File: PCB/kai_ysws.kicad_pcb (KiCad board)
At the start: 4 copper layers, 22 x 42 mm, 163 parts, among them J1 Bus_M.2_Socket_M, U1 24C02Cx-x-MNY, U2 AP2112K-3.3, U3 AP2112K-1.8, U4 RP23534A, U5 CH382L, Y1 22.1184MHz, Y2 ABM8-272-T3

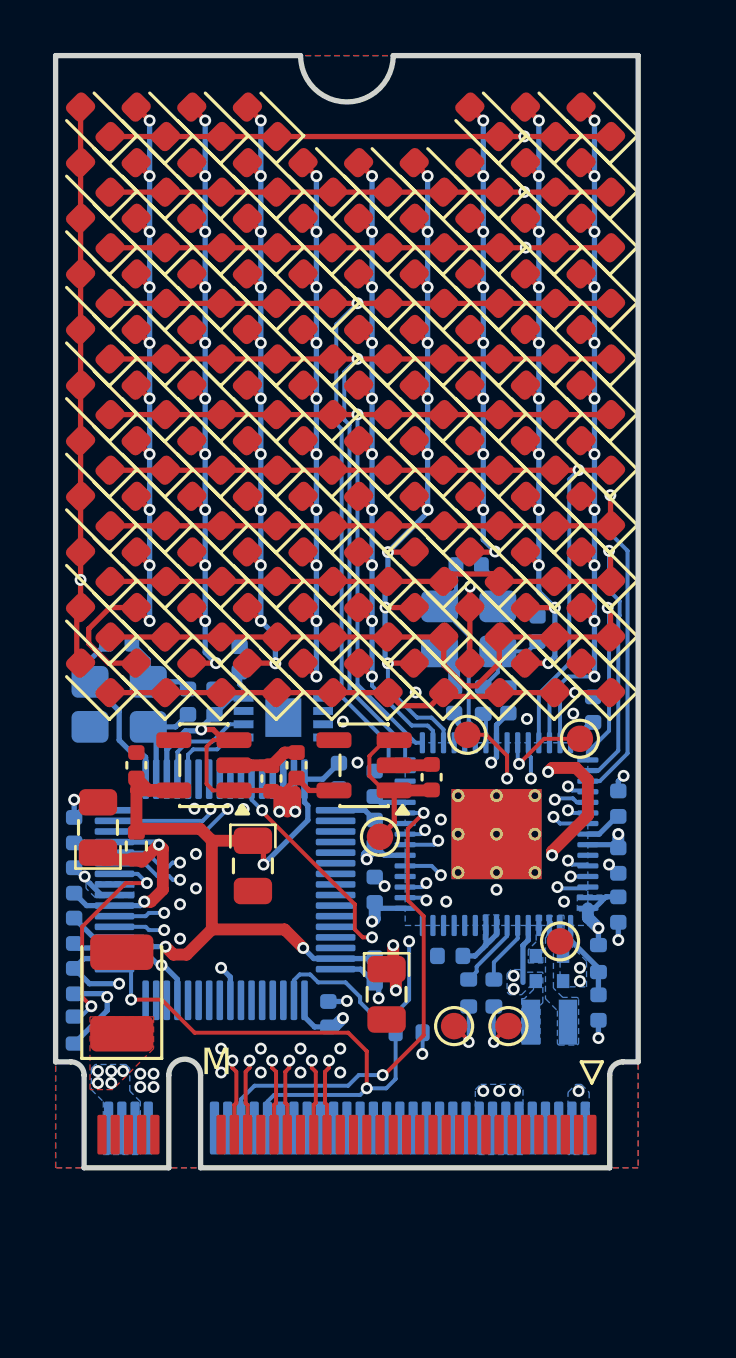
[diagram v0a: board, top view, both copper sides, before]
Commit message: fixed Bom again and small pcb things
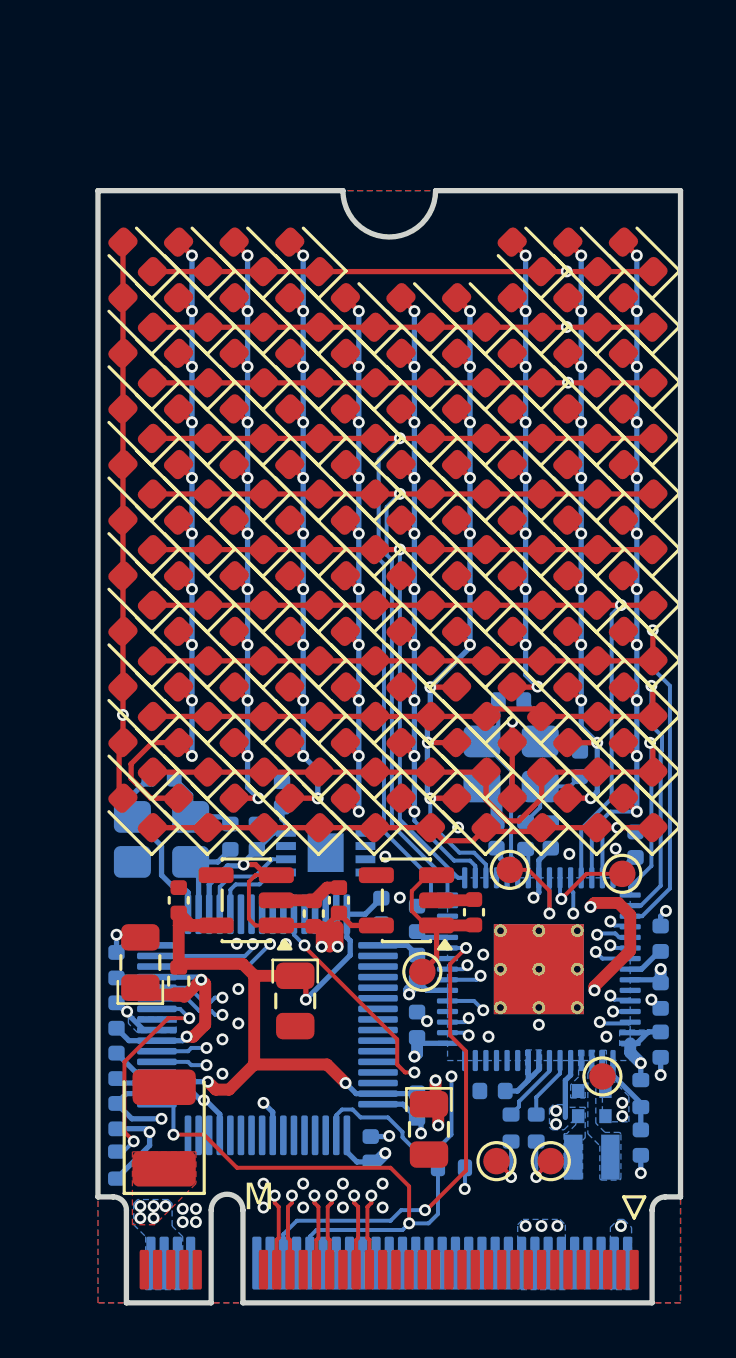
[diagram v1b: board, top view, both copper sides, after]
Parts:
- moved C32 5.35 mm to (135.3, 119.7)
- moved D29 5.35 mm to (133.3, 101.7)
- moved D49 5.35 mm to (133.3, 105.9)
- moved D79 5.35 mm to (133.3, 112.2)
- moved D99 5.35 mm to (133.3, 116.4)
- moved R5 5.35 mm to (131.6, 130.4)
- moved TP2 5.35 mm to (130.1, 131.7)
- moved TP5 5.35 mm to (130.6, 120.7)
- moved C10 5.35 mm to (125.7, 122.2)
- moved C11 5.35 mm to (115.7, 126.2)
- moved C2 5.35 mm to (117.4, 117.2)
- moved C9 5.35 mm to (115.7, 128.1)
- moved D23 5.35 mm to (120.7, 101.7)
- moved D25 5.35 mm to (124.9, 101.7)
- moved D43 5.35 mm to (120.7, 105.9)
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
